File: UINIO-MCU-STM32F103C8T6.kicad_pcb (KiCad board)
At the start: 2 copper layers, 68.4 x 20.3 mm, 41 parts, among them J1 Conn_01x24_Pin, J2 Conn_01x24_Pin, J3 Conn_01x04_Pin, SW1 BOOT1, SW2 NRST, SW3 BOOT0, U1 ME6211C33M5G-N, U2 GD32F103C8T6, Y1 32.768KHz, Y2 8MHz

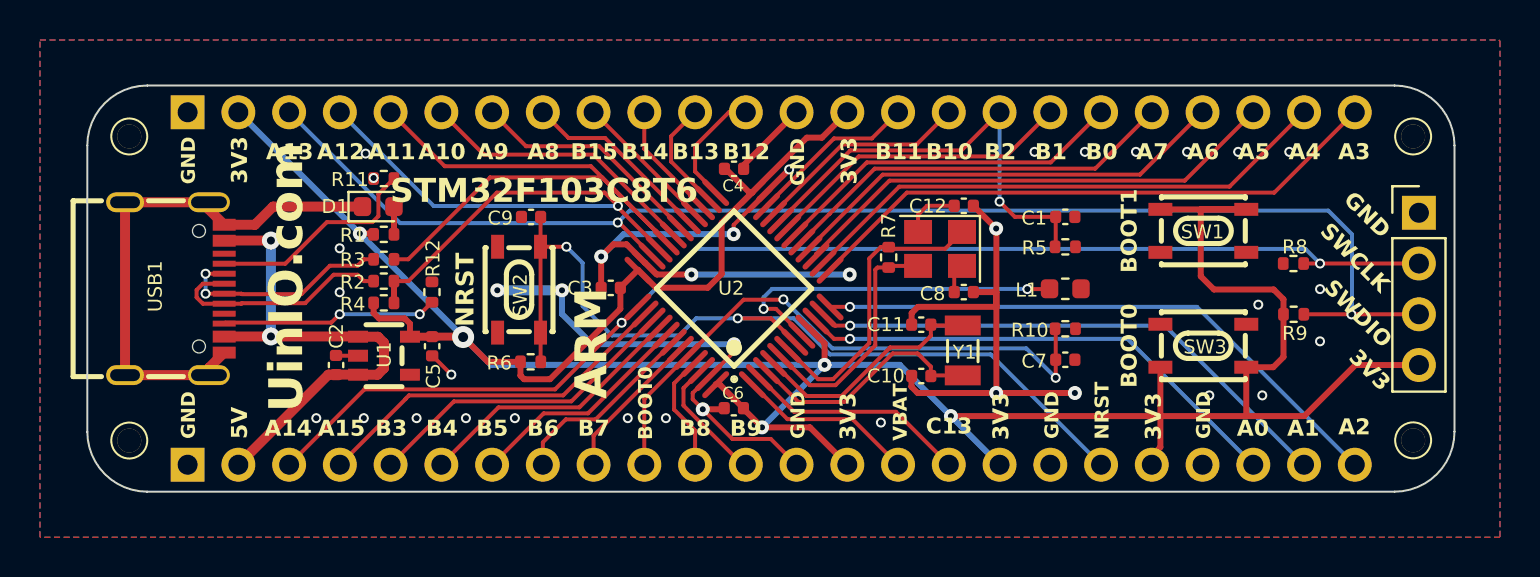
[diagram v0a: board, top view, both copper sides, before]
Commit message: Complete wiring.
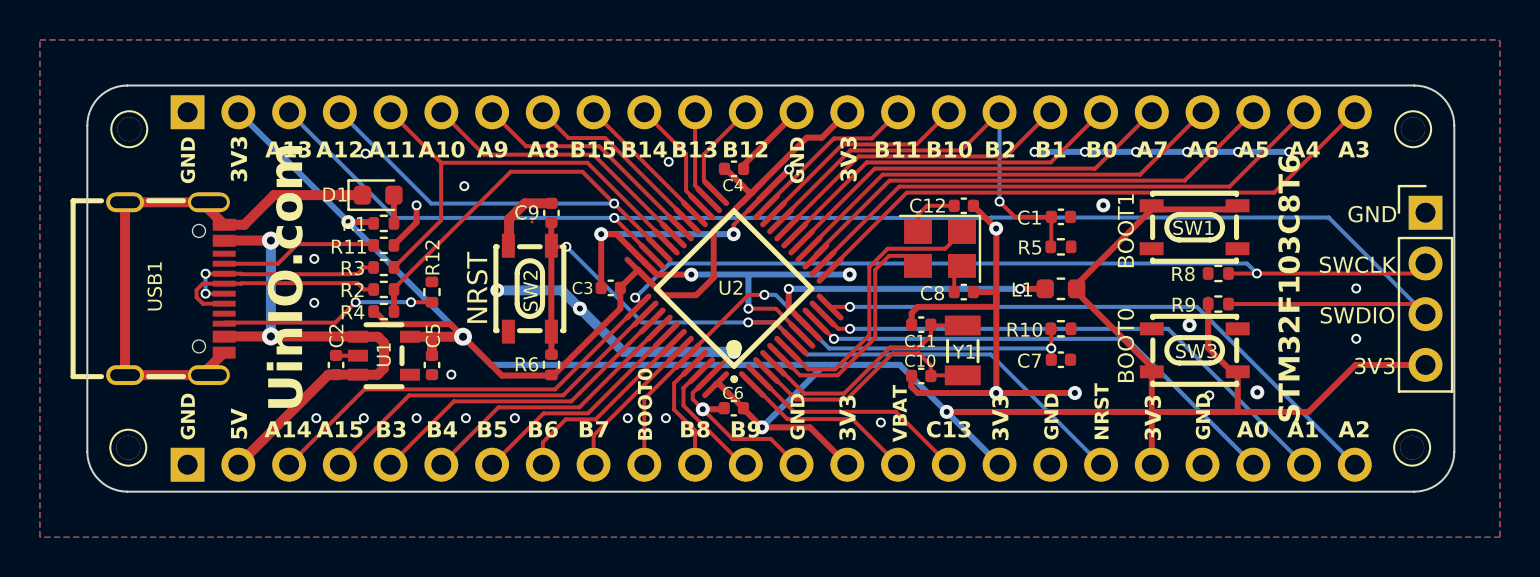
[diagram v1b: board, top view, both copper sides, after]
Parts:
- removed R7: 1M, Resistor_SMD:R_0402_1005Metric
- C12, C8: value 20pF -> 22pF
- U2: value GD32F103C8T6 -> STM32F103C8T6
- moved R9 3.80 mm to (173.9, 100.6)
- moved R8 3.79 mm to (173.9, 99.1)
- moved R11 3.35 mm to (132.2, 97.7), turned to 0 degrees
- moved R6 1.05 mm to (140.5, 103.7), turned to 90 degrees
- moved C9 1.04 mm to (140.5, 96.0), turned to 90 degrees
- moved C5 0.94 mm to (134.6, 103.7)
- moved D1 0.57 mm to (131.9, 95.2)
- moved R1 0.55 mm to (132.1, 96.6)
- moved SW2 0.54 mm to (139.5, 99.8)
- moved SW3 0.49 mm to (172.7, 102.9)
- moved SW1 0.47 mm to (172.7, 96.8)
- moved R4 0.43 mm to (132.2, 101.0)
- moved R2 0.42 mm to (132.2, 99.9), turned to 0 degrees
- moved R3 0.41 mm to (132.2, 98.8), turned to 0 degrees
- moved HOLE** 0.37 mm to (183.6, 107.8)
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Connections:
- L1 pad 1: GND -> /VDD_3.3V
- L1 pad 2: Net-(U2-VSSA) -> Net-(U2-VDDA)
- R2 pad 1: /PA12 -> /USB_Data+
- R2 pad 2: /USB_Data+ -> /PA12
- R3 pad 1: /PA11 -> /USB_Data-
- R3 pad 2: /USB_Data- -> /PA11
- U2 pad 8: Net-(U2-VSSA) -> GND
- U2 pad 9: /VDD_3.3V -> Net-(U2-VDDA)
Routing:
- net GND: track 110.2 -> 132.6 mm, vias 36 -> 40
- net Net-(U2-VSSA): track 17.5 -> 0.00 mm, vias 2 -> 0
- net Net-(U2-VDDA): track 0.00 -> 15.5 mm, vias 0 -> 2
- net /PA11: track 33.1 -> 22.7 mm
- net /PA13/SWDIO: track 68.4 -> 73.0 mm, vias 2 -> 1
- net /NRST: track 45.0 -> 41.4 mm
- net Net-(USB1-CC1): track 10.9 -> 7.89 mm
- net /VDD_3.3V: track 148.6 -> 150.3 mm, vias 5 -> 4
- net /BOOT0: track 30.0 -> 28.5 mm
- net /PB13: track 5.62 -> 4.62 mm
- net /PA14/SWCLK: track 63.3 -> 62.4 mm
- net /PB12: track 5.97 -> 5.10 mm
- net Net-(U2-PD1_OSC_OUT): track 14.8 -> 14.0 mm
- net /PA12: track 33.3 -> 34.0 mm
- net /USB_Data+: track 11.6 -> 11.0 mm
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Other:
- outline, holes or cut-outs redrawn
- board text added: "Version 3.0.0"
- board text removed: "ARM"
- board text removed: "Version 2.0.0"
